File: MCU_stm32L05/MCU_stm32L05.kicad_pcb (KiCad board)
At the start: 2 copper layers, 7 parts, among them SW1 SW_SPDT, U1 STM32L052K6Tx, U2 AP2210K-3.3TRG1, Y1 32.768kHz

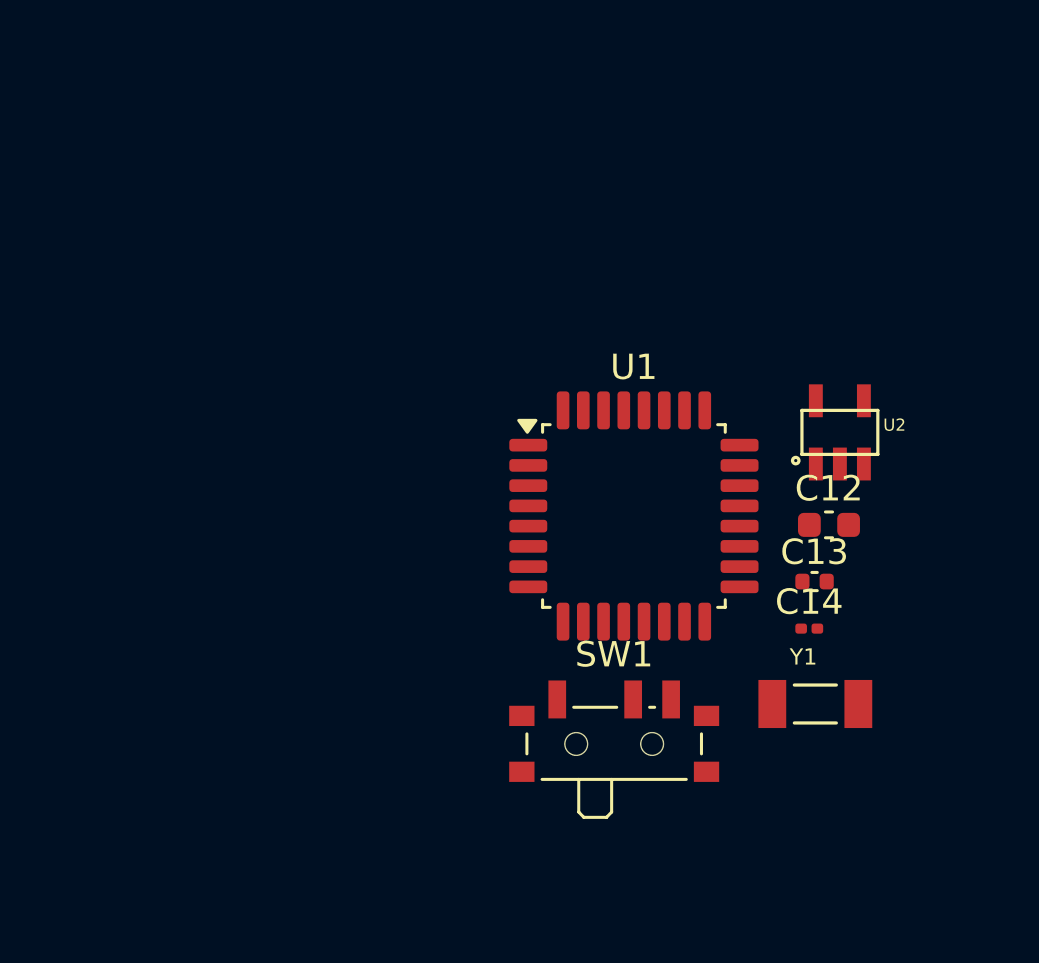
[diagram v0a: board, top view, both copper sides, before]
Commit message: update
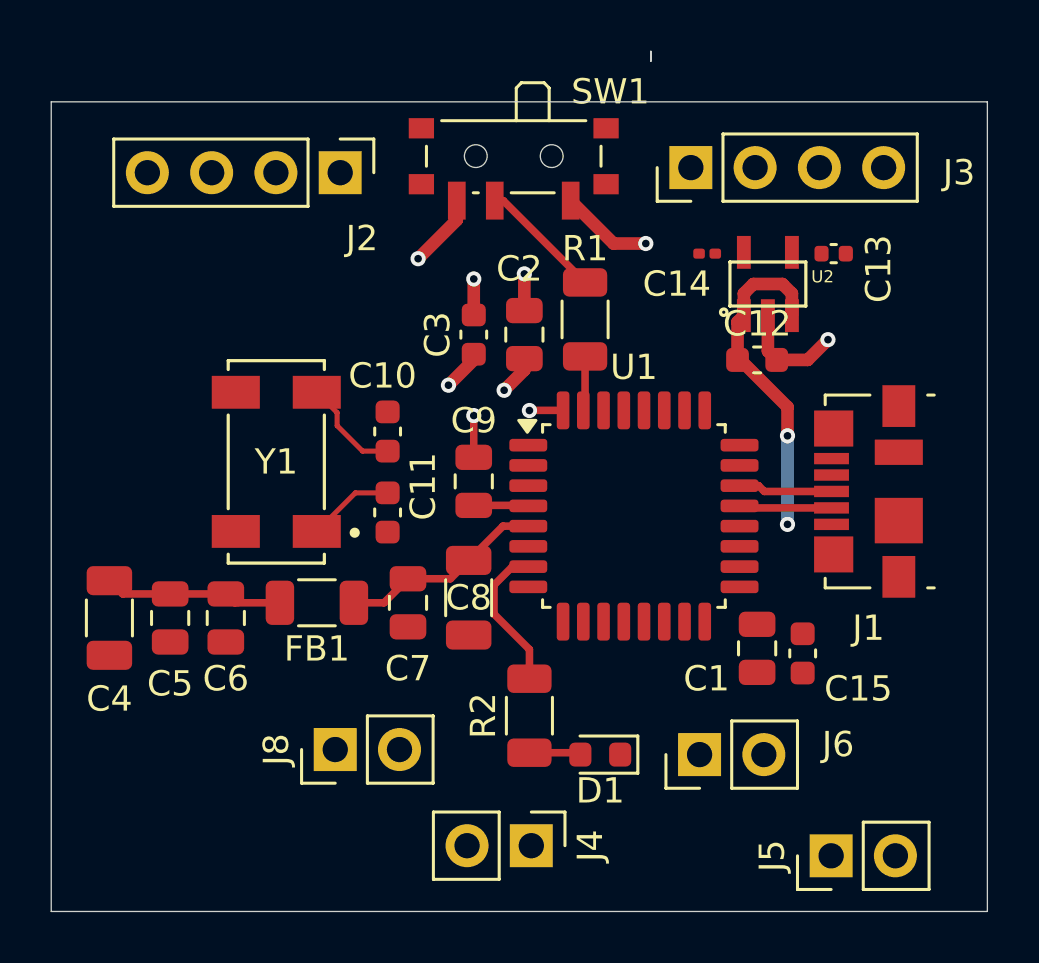
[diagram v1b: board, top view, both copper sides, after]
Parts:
- added C1: 0.1u, Capacitor_SMD:C_0805_2012Metric, F.Cu at (70.0, 60.0)
- added C10: 10p, Capacitor_SMD:C_0603_1608Metric, F.Cu at (55.4, 51.4)
- added C11: 10p, Capacitor_SMD:C_0603_1608Metric, F.Cu at (55.4, 54.6)
- added C15: 10u, Capacitor_SMD:C_0603_1608Metric, F.Cu at (71.8, 60.2)
- added C2: 0.1u, Capacitor_SMD:C_0805_2012Metric, F.Cu at (60.8, 47.6)
- added C3: 10u, Capacitor_SMD:C_0603_1608Metric, F.Cu at (58.8, 47.6)
- added C4: 4.7u, Capacitor_SMD:C_1206_3216Metric, F.Cu at (44.4, 58.8)
- added C5: 0.1u, Capacitor_SMD:C_0805_2012Metric, F.Cu at (46.8, 58.8)
- added C6: 0.1u, Capacitor_SMD:C_0805_2012Metric, F.Cu at (49.0, 58.8)
- added C7: 1u, Capacitor_SMD:C_0805_2012Metric, F.Cu at (56.2, 58.2)
- added C8: 10n, Capacitor_SMD:C_1206_3216Metric, F.Cu at (58.6, 58.0)
- added C9: 0.1u, Capacitor_SMD:C_0805_2012Metric, F.Cu at (58.8, 53.4)
- added D1: LED, LED_SMD:LED_0603_1608Metric, F.Cu at (63.8, 64.2)
- added FB1: 600R, Resistor_SMD:R_1206_3216Metric, F.Cu at (52.6, 58.2)
- added J1: USB_B_Micro, Connector_USB:USB_Micro-B_Molex_47346-0001, F.Cu at (74.4, 53.8)
- added J2: Conn_01x04, Connector_PinHeader_2.54mm:PinHeader_1x04_P2.54mm_Vertical, F.Cu at (53.5, 41.2)
- added J3: Conn_01x04, Connector_PinHeader_2.54mm:PinHeader_1x04_P2.54mm_Vertical, F.Cu at (67.4, 41.0)
- added J4: Conn_01x02, Connector_PinHeader_2.54mm:PinHeader_1x02_P2.54mm_Vertical, F.Cu at (61.1, 67.8)
- added J5: Conn_01x02, Connector_PinHeader_2.54mm:PinHeader_1x02_P2.54mm_Vertical, F.Cu at (72.9, 68.2)
- added J6: Conn_01x02, Connector_PinHeader_2.54mm:PinHeader_1x02_P2.54mm_Vertical, F.Cu at (67.7, 64.2)
- added J8: Conn_01x02, Connector_PinHeader_2.54mm:PinHeader_1x02_P2.54mm_Vertical, F.Cu at (53.3, 64.0)
- added R1: 10k, Resistor_SMD:R_1206_3216Metric, F.Cu at (63.2, 47.0)
- added R2: 10k, Resistor_SMD:R_1206_3216Metric, F.Cu at (61.0, 62.7)
- Y1: footprint crystal:XTAL_CC5V-T1A_32.768KHZ_12.5PF_20PPM_TA_QC -> crystal:XTAL_ABS25-32.768KHZ-6-T
- moved Y1 23.4 mm to (51.0, 52.6), turned to 180 degrees
- moved SW1 22.9 mm to (60.4, 40.9), turned to 180 degrees
- moved C14 15.4 mm to (68.0, 44.4), turned to 180 degrees
- moved C13 13.0 mm to (73.0, 44.4)
- moved C12 7.11 mm to (70.0, 48.6)
- moved U2 6.52 mm to (70.4, 45.6)
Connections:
- U1 pad 1: GND -> +3.3V
- U1 pad 17: GND -> +3.3V
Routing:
- net GND: track 0.00 -> 13.8 mm, vias 0 -> 6
- net +3.3V: track 0.00 -> 13.2 mm, vias 0 -> 3
- net VBUS: track 0.00 -> 13.2 mm, vias 0 -> 2
- net +3.3VA: track 0.00 -> 8.15 mm
- net /PWR_LED: track 0.00 -> 5.94 mm
- net Net-(SW1-B): track 0.00 -> 5.25 mm
- net /OSC_IN: track 0.00 -> 4.06 mm
- net /USB_DM+: track 0.00 -> 3.73 mm
- net /USB_DP-: track 0.00 -> 3.67 mm
- net /OSC_OUT: track 0.00 -> 3.43 mm
- net /NRST: track 0.00 -> 2.16 mm
- net /BOOT0: track 0.00 -> 2.16 mm
- net Net-(D1-A): track 0.00 -> 2.04 mm
- added copper zone on In2.Cu, net +3.3V
- added copper zone on In1.Cu, net GND
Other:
- board outline added: 37 x 34 mm
- copper layers 2 -> 4

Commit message: update
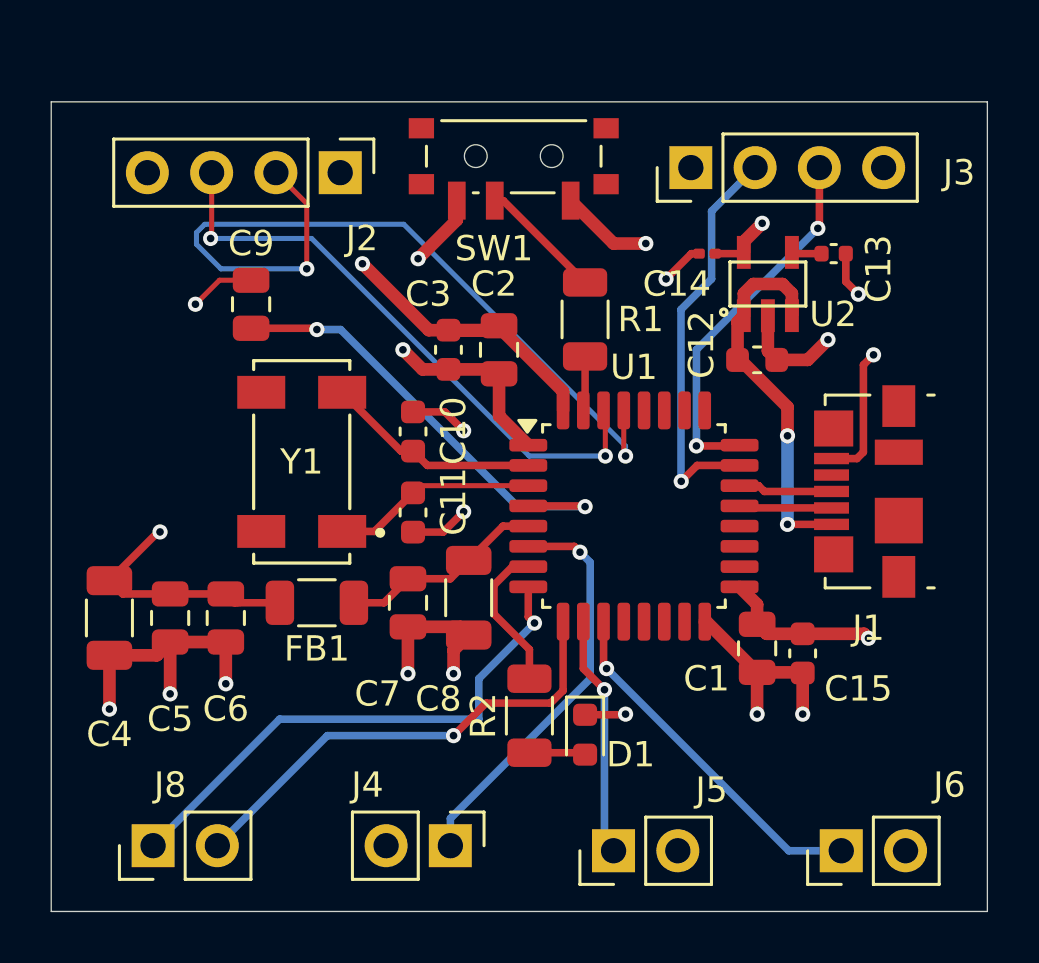
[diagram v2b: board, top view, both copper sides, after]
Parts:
- moved C9 11.2 mm to (50.0, 46.4)
- moved J5 8.60 mm to (64.3, 68.0)
- moved J8 8.14 mm to (46.1, 67.8)
- moved J6 6.77 mm to (73.3, 68.0)
- moved J4 3.20 mm to (57.9, 67.8)
- moved C2 1.17 mm to (59.8, 48.2)
- moved C3 1.17 mm to (57.8, 48.2)
- moved Y1 1.01 mm to (52.0, 52.6)
- moved C10 1.00 mm to (56.4, 51.4)
- moved C11 1.00 mm to (56.4, 54.6)
- moved D1 0.99 mm to (63.2, 63.4), turned to -90 degrees
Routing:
- net GND: track 13.8 -> 63.3 mm, vias 6 -> 17
- net /I2C_SCL: track 0.00 -> 32.5 mm, vias 0 -> 2
- net /I2C_SDA: track 0.00 -> 23.6 mm, vias 0 -> 2
- net /TX: track 0.00 -> 21.2 mm, vias 0 -> 1
- net /RX: track 0.00 -> 18.9 mm, vias 0 -> 1
- net /NRST: track 2.16 -> 18.4 mm, vias 0 -> 2
- net /ADC_IN0: track 0.00 -> 16.2 mm, vias 0 -> 1
- net /SWDIO: track 0.00 -> 16.2 mm, vias 0 -> 1
- net +3.3V: track 13.2 -> 29.3 mm, vias 3 -> 5
- net /SWCLK: track 0.00 -> 14.7 mm, vias 0 -> 2
- net /ADC_IN5: track 0.00 -> 14.2 mm, vias 0 -> 1
- net /ADC_IN4: track 0.00 -> 9.55 mm, vias 0 -> 1
- net /OSC_OUT: track 3.43 -> 8.13 mm
- net /OSC_IN: track 4.06 -> 8.55 mm
- net VBUS: track 13.2 -> 14.9 mm
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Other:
- board size 37 x 34 mm -> 37 x 32 mm
